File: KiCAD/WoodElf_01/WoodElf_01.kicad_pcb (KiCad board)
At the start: 2 copper layers, 154.3 x 119.4 mm, 164 parts, among them J1 AnalogJoystick, P1 ItsyBitsyM4Express

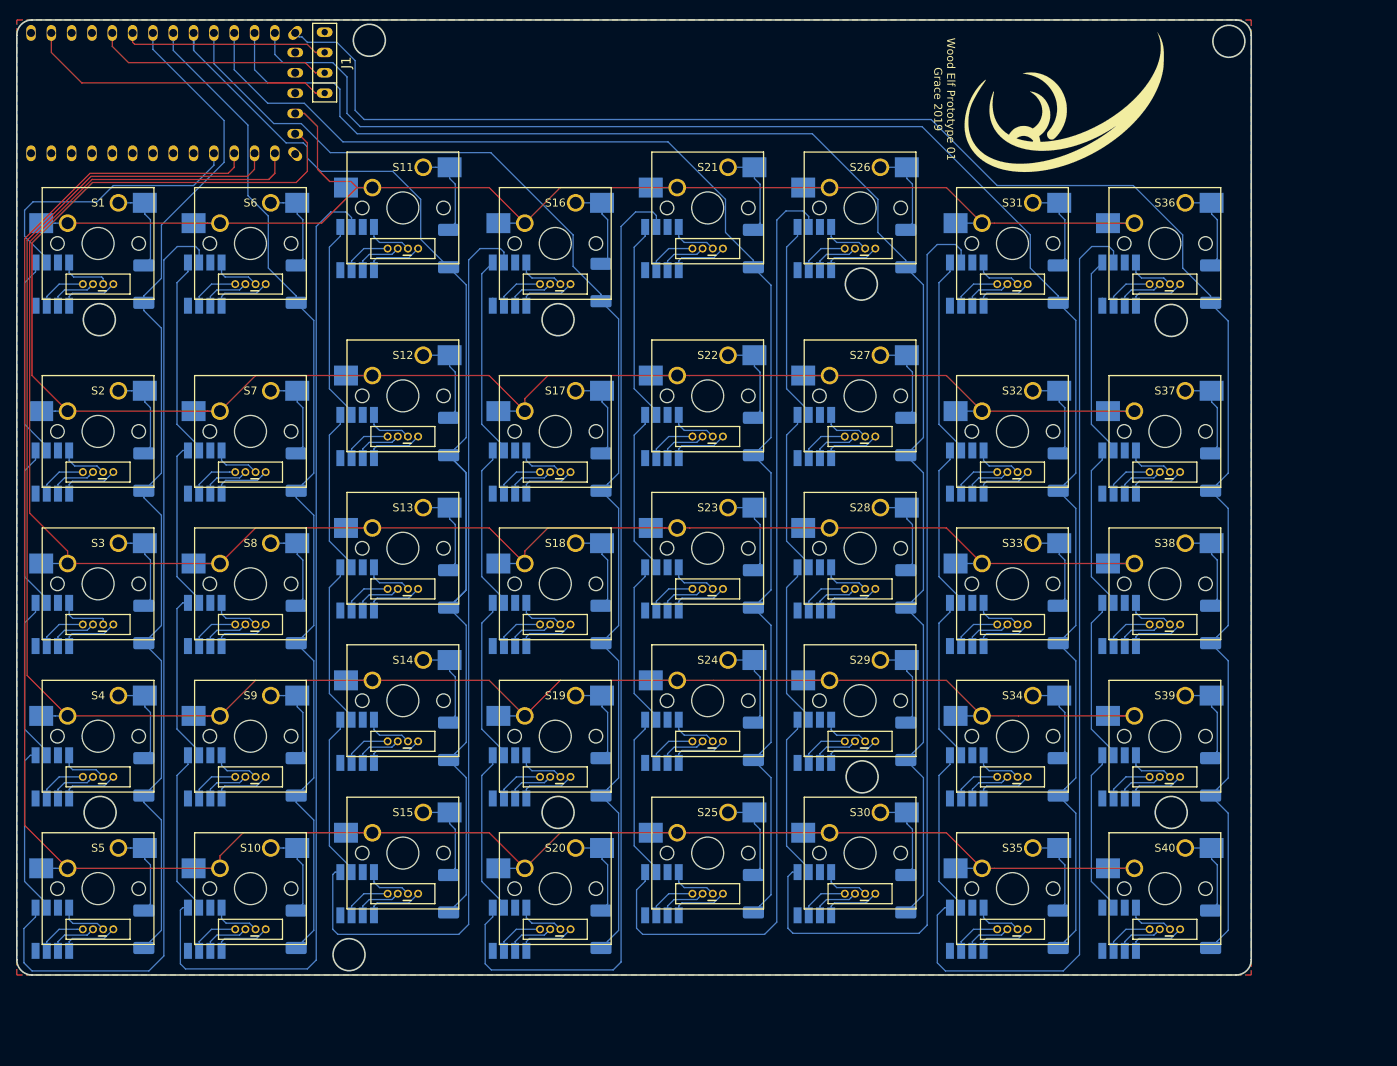
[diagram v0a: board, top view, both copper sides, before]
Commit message: Started on a full-size PCB
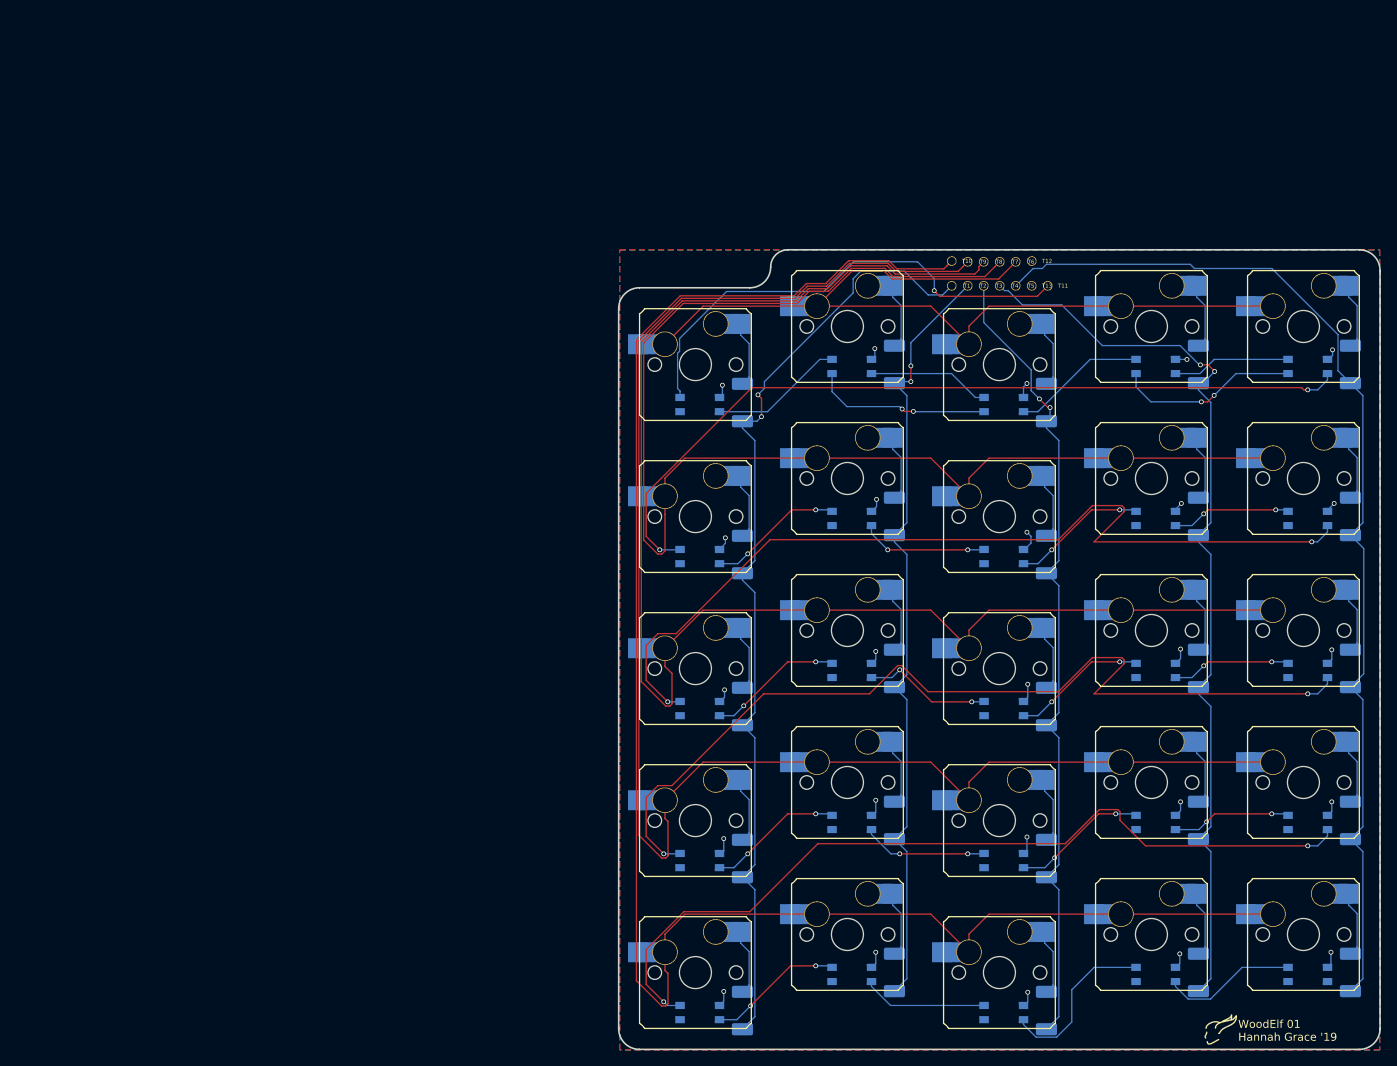
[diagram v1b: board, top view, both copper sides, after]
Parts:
- removed C1, C10, C11, C12, C13, C14, C15, C16, C17, C18, C19, C2, C20, C21, C22, C23, C24, C25, C26, C27, C28, C29, C3, C30, C31, C32, C33, C34, C35, C36, C37, C38, C39, C4, C40, C5, C6, C7, C8, C9: WS2811, WoodElfLib:WS2811
- removed D26, D27, D28, D29, D30, D31, D32, D33, D34, D35, D36, D37, D38, D39, D40: D, Diode_SMD:D_2010_5025Metric_Pad1.52x2.65mm_HandSolder
- removed H26, H27, H28, H29, H30, H31, H32, H33, H34, H35, H36, H37, H38, H39, H40: Kailh_HotSwap_SwitchMount, WoodElfLib:Kailh_HotSwap_Socket
- removed J1: AnalogJoystick, WoodElfLib:Joystick
- removed Logo_2 (x2): Wood Elf, WoodElfLib:WoodElfLogo
- removed P1: ItsyBitsyM4Express, WoodElfLib:ItsyBitsyM4Express
- removed S26, S27, S28, S29, S30, S31, S32, S33, S34, S35, S36, S37, S38, S39, S40: Kailh_RGB_Switch, WoodElfLib:SW_Cherry_MX1A_1.00u_PCB
- added G***: Tiefling_Logo, WoodElf_Lib:Tiefling_Logo, F.Cu at (174.6, 151.2)
- added L1: SK6812MINI, WoodElf_Lib:LED_SK6812MINI_PLCC4_3.5x3.5mm_P1.75mm, F.Cu at (109.5, 72.8)
- added L10: SK6812MINI, WoodElf_Lib:LED_SK6812MINI_PLCC4_3.5x3.5mm_P1.75mm, F.Cu at (109.5, 91.8)
- added L11: SK6812MINI, WoodElf_Lib:LED_SK6812MINI_PLCC4_3.5x3.5mm_P1.75mm, F.Cu at (109.5, 110.8)
- added L12: SK6812MINI, WoodElf_Lib:LED_SK6812MINI_PLCC4_3.5x3.5mm_P1.75mm, F.Cu at (128.5, 106.1)
- added L13: SK6812MINI, WoodElf_Lib:LED_SK6812MINI_PLCC4_3.5x3.5mm_P1.75mm, F.Cu at (147.5, 110.8)
- added L14: SK6812MINI, WoodElf_Lib:LED_SK6812MINI_PLCC4_3.5x3.5mm_P1.75mm, F.Cu at (166.5, 106.1)
- added L15: SK6812MINI, WoodElf_Lib:LED_SK6812MINI_PLCC4_3.5x3.5mm_P1.75mm, F.Cu at (185.5, 106.1)
- added L16: SK6812MINI, WoodElf_Lib:LED_SK6812MINI_PLCC4_3.5x3.5mm_P1.75mm, F.Cu at (185.5, 125.1)
- added L17: SK6812MINI, WoodElf_Lib:LED_SK6812MINI_PLCC4_3.5x3.5mm_P1.75mm, F.Cu at (166.5, 125.1)
- added L18: SK6812MINI, WoodElf_Lib:LED_SK6812MINI_PLCC4_3.5x3.5mm_P1.75mm, F.Cu at (147.5, 129.8)
- added L19: SK6812MINI, WoodElf_Lib:LED_SK6812MINI_PLCC4_3.5x3.5mm_P1.75mm, F.Cu at (128.5, 125.1)
- added L2: SK6812MINI, WoodElf_Lib:LED_SK6812MINI_PLCC4_3.5x3.5mm_P1.75mm, F.Cu at (128.5, 68.1)
- added L20: SK6812MINI, WoodElf_Lib:LED_SK6812MINI_PLCC4_3.5x3.5mm_P1.75mm, F.Cu at (109.5, 129.8)
- added L21: SK6812MINI, WoodElf_Lib:LED_SK6812MINI_PLCC4_3.5x3.5mm_P1.75mm, F.Cu at (109.5, 148.8)
- added L22: SK6812MINI, WoodElf_Lib:LED_SK6812MINI_PLCC4_3.5x3.5mm_P1.75mm, F.Cu at (128.5, 144.1)
- added L23: SK6812MINI, WoodElf_Lib:LED_SK6812MINI_PLCC4_3.5x3.5mm_P1.75mm, F.Cu at (147.5, 148.8)
- added L24: SK6812MINI, WoodElf_Lib:LED_SK6812MINI_PLCC4_3.5x3.5mm_P1.75mm, F.Cu at (166.5, 144.1)
- added L25: SK6812MINI, WoodElf_Lib:LED_SK6812MINI_PLCC4_3.5x3.5mm_P1.75mm, F.Cu at (185.5, 144.1)
- added L3: SK6812MINI, WoodElf_Lib:LED_SK6812MINI_PLCC4_3.5x3.5mm_P1.75mm, F.Cu at (147.5, 72.8)
- added L4: SK6812MINI, WoodElf_Lib:LED_SK6812MINI_PLCC4_3.5x3.5mm_P1.75mm, F.Cu at (166.5, 68.1)
- added L5: SK6812MINI, WoodElf_Lib:LED_SK6812MINI_PLCC4_3.5x3.5mm_P1.75mm, F.Cu at (185.5, 68.1)
- added L6: SK6812MINI, WoodElf_Lib:LED_SK6812MINI_PLCC4_3.5x3.5mm_P1.75mm, F.Cu at (185.5, 87.1)
- added L7: SK6812MINI, WoodElf_Lib:LED_SK6812MINI_PLCC4_3.5x3.5mm_P1.75mm, F.Cu at (166.5, 87.1)
- added L8: SK6812MINI, WoodElf_Lib:LED_SK6812MINI_PLCC4_3.5x3.5mm_P1.75mm, F.Cu at (147.5, 91.8)
- added L9: SK6812MINI, WoodElf_Lib:LED_SK6812MINI_PLCC4_3.5x3.5mm_P1.75mm, F.Cu at (128.5, 87.1)
- added T1: BlankThrough-Hole, WoodElf_Lib:BlankThrough-Hole, F.Cu at (141.0, 58.0)
- added T10: BlankThrough-Hole, WoodElf_Lib:BlankThrough-Hole, F.Cu at (141.0, 54.9)
- added T11: BlankThrough-Hole, WoodElf_Lib:BlankThrough-Hole, F.Cu at (153.0, 58.0)
- added T12: BlankThrough-Hole, WoodElf_Lib:BlankThrough-Hole, F.Cu at (151.0, 54.9)
- added T13: BlankThrough-Hole, WoodElf_Lib:BlankThrough-Hole, F.Cu at (151.0, 58.0)
- added T2: BlankThrough-Hole, WoodElf_Lib:BlankThrough-Hole, F.Cu at (143.0, 58.0)
- added T3: BlankThrough-Hole, WoodElf_Lib:BlankThrough-Hole, F.Cu at (145.0, 58.0)
- added T4: BlankThrough-Hole, WoodElf_Lib:BlankThrough-Hole, F.Cu at (147.0, 58.0)
- added T5: BlankThrough-Hole, WoodElf_Lib:BlankThrough-Hole, F.Cu at (149.0, 58.0)
- added T6: BlankThrough-Hole, WoodElf_Lib:BlankThrough-Hole, F.Cu at (149.0, 55.0)
- added T7: BlankThrough-Hole, WoodElf_Lib:BlankThrough-Hole, F.Cu at (147.0, 55.0)
- added T8: BlankThrough-Hole, WoodElf_Lib:BlankThrough-Hole, F.Cu at (145.0, 55.0)
- added T9: BlankThrough-Hole, WoodElf_Lib:BlankThrough-Hole, F.Cu at (143.0, 55.0)
- D1, D10, D11, D12, D13, D14, D15, D16, D17, D18, D19, D2, D20, D21, D22, D23, D24, D25, D3, D4, D5, D6, D7, D8, D9: value D -> DIODE; footprint WoodElfLib:D_2010_5025Metric_Pad1.52x2.65mm_HandSolder -> Diode_SMD:D_2010_5025Metric_Pad1.52x2.65mm_HandSolder
- H1, H10, H11, H12, H13, H14, H15, H16, H17, H18, H19, H2, H20, H21, H22, H23, H24, H25, H3, H4, H5, H6, H7, H8, H9: footprint WoodElfLib:Kailh_HotSwap_Socket -> WoodElf_Lib:Kailh_HotSwap_Socket
- S1, S10, S11, S12, S13, S14, S15, S16, S17, S18, S19, S2, S20, S21, S22, S23, S24, S25, S3, S4, S5, S6, S7, S8, S9: footprint WoodElfLib:SW_Cherry_MX1A_1.00u_PCB -> WoodElf_Lib:SW_Cherry_MX1A_1.00u_PCB
- moved D5 166.5 mm to (190.8, 67.8), turned to 270 degrees
- moved H5 166.3 mm to (187.5, 58.0)
- moved S5 166.3 mm to (187.5, 58.0)
- moved D4 141.6 mm to (171.8, 67.8), turned to 270 degrees
- moved H4 141.3 mm to (168.5, 58.0)
- moved S4 141.3 mm to (168.5, 58.0)
- moved D6 134.9 mm to (190.8, 86.8), turned to 270 degrees
- moved H6 134.9 mm to (187.5, 77.0)
- moved S6 134.9 mm to (187.5, 77.0)
- moved D15 116.2 mm to (190.8, 105.8), turned to 270 degrees
- moved D3 116.2 mm to (152.8, 72.6), turned to 270 degrees
- moved H15 116.0 mm to (187.5, 96.0)
- moved S15 116.0 mm to (187.5, 96.0)
- moved H3 116.0 mm to (149.5, 62.8)
- moved S3 116.0 mm to (149.5, 62.8)
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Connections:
- D1 pad 1: /A2 -> Net-(D1-Pad1)
- D1 pad 2: Net-(D1-Pad2) -> /Col2
- D10 pad 1: /A3 -> Net-(D10-Pad1)
- D10 pad 2: Net-(D10-Pad2) -> /Col1
- D11 pad 1: /A4 -> Net-(D11-Pad1)
- D11 pad 2: Net-(D11-Pad2) -> /Col1
- D12 pad 1: /A4 -> Net-(D12-Pad1)
- D12 pad 2: Net-(D12-Pad2) -> /Col2
- D13 pad 1: /A4 -> Net-(D13-Pad1)
- D13 pad 2: Net-(D13-Pad2) -> /Col3
- D14 pad 1: /A4 -> Net-(D14-Pad1)
- D14 pad 2: Net-(D14-Pad2) -> /Col4
- D15 pad 1: /A4 -> Net-(D15-Pad1)
- D15 pad 2: Net-(D15-Pad2) -> /Col5
- D16 pad 1: /A5 -> Net-(D16-Pad1)
- D16 pad 2: Net-(D16-Pad2) -> /Col5
- D17 pad 1: /A5 -> Net-(D17-Pad1)
- D17 pad 2: Net-(D17-Pad2) -> /Col4
- D18 pad 1: /A5 -> Net-(D18-Pad1)
- D18 pad 2: Net-(D18-Pad2) -> /Col3
- D19 pad 1: /A5 -> Net-(D19-Pad1)
- D19 pad 2: Net-(D19-Pad2) -> /Col2
- D2 pad 1: /A2 -> Net-(D2-Pad1)
- D2 pad 2: Net-(D2-Pad2) -> /Col1
- D20 pad 1: /A5 -> Net-(D20-Pad1)
- D20 pad 2: Net-(D20-Pad2) -> /Col1
- D21 pad 1: /SCK -> Net-(D21-Pad1)
- D21 pad 2: Net-(D21-Pad2) -> /Col1
- D22 pad 1: /SCK -> Net-(D22-Pad1)
- D22 pad 2: Net-(D22-Pad2) -> /Col2
- D23 pad 1: /SCK -> Net-(D23-Pad1)
- D23 pad 2: Net-(D23-Pad2) -> /Col3
- D24 pad 1: /SCK -> Net-(D24-Pad1)
- D24 pad 2: Net-(D24-Pad2) -> /Col4
- D25 pad 1: /SCK -> Net-(D25-Pad1)
- D25 pad 2: Net-(D25-Pad2) -> /Col5
- D3 pad 1: /A2 -> Net-(D3-Pad1)
- D3 pad 2: Net-(D3-Pad2) -> /Col3
- D4 pad 1: /A2 -> Net-(D4-Pad1)
- D4 pad 2: Net-(D4-Pad2) -> /Col4
- D5 pad 1: /A2 -> Net-(D5-Pad1)
- D5 pad 2: Net-(D5-Pad2) -> /Col5
- D6 pad 1: /A3 -> Net-(D6-Pad1)
- D6 pad 2: Net-(D6-Pad2) -> /Col5
- D7 pad 1: /A3 -> Net-(D7-Pad1)
- D7 pad 2: Net-(D7-Pad2) -> /Col4
- D8 pad 1: /A3 -> Net-(D8-Pad1)
- D8 pad 2: Net-(D8-Pad2) -> /Col3
- D9 pad 1: /A3 -> Net-(D9-Pad1)
- D9 pad 2: Net-(D9-Pad2) -> /Col2
- H1 pad 1: Net-(D2-Pad2) -> Net-(D2-Pad1)
- H1 pad 2: /GPIO#3 -> /Row1
- H10 pad 1: Net-(D10-Pad2) -> Net-(D10-Pad1)
- H10 pad 2: /SCL -> /Row2
- H11 pad 1: Net-(D11-Pad2) -> Net-(D11-Pad1)
- H11 pad 2: /GPIO#3 -> /Row3
- H12 pad 1: Net-(D12-Pad2) -> Net-(D12-Pad1)
- H12 pad 2: /GPIO#4 -> /Row3
- H13 pad 1: Net-(D13-Pad2) -> Net-(D13-Pad1)
- H13 pad 2: /GPIO#1 -> /Row3
- H14 pad 1: Net-(D14-Pad2) -> Net-(D14-Pad1)
- H14 pad 2: /SDA -> /Row3
- H15 pad 1: Net-(D15-Pad2) -> Net-(D15-Pad1)
- H15 pad 2: /SCL -> /Row3
- H16 pad 1: Net-(D16-Pad2) -> Net-(D16-Pad1)
- H16 pad 2: /GPIO#3 -> /Row4
- H17 pad 1: Net-(D17-Pad2) -> Net-(D17-Pad1)
- H17 pad 2: /GPIO#4 -> /Row4
- H18 pad 1: Net-(D18-Pad2) -> Net-(D18-Pad1)
- H18 pad 2: /GPIO#1 -> /Row4
- H19 pad 1: Net-(D19-Pad2) -> Net-(D19-Pad1)
- H19 pad 2: /SDA -> /Row4
- H2 pad 1: Net-(D1-Pad2) -> Net-(D1-Pad1)
- H2 pad 2: /GPIO#4 -> /Row1
- H20 pad 1: Net-(D20-Pad2) -> Net-(D20-Pad1)
- H20 pad 2: /SCL -> /Row4
- H21 pad 1: Net-(D21-Pad2) -> Net-(D21-Pad1)
- H21 pad 2: /GPIO#3 -> /Row5
- H22 pad 1: Net-(D22-Pad2) -> Net-(D22-Pad1)
- H22 pad 2: /GPIO#4 -> /Row5
- H23 pad 1: Net-(D23-Pad2) -> Net-(D23-Pad1)
- H23 pad 2: /GPIO#1 -> /Row5
- H24 pad 1: Net-(D24-Pad2) -> Net-(D24-Pad1)
- H24 pad 2: /SDA -> /Row5
- H25 pad 1: Net-(D25-Pad2) -> Net-(D25-Pad1)
- H25 pad 2: /SCL -> /Row5
- H3 pad 1: Net-(D3-Pad2) -> Net-(D3-Pad1)
- H3 pad 2: /GPIO#1 -> /Row1
- H4 pad 1: Net-(D4-Pad2) -> Net-(D4-Pad1)
- H4 pad 2: /SDA -> /Row1
- H5 pad 1: Net-(D5-Pad2) -> Net-(D5-Pad1)
- H5 pad 2: /SCL -> /Row1
- H6 pad 1: Net-(D6-Pad2) -> Net-(D6-Pad1)
- H6 pad 2: /GPIO#3 -> /Row2
- H7 pad 1: Net-(D7-Pad2) -> Net-(D7-Pad1)
- H7 pad 2: /GPIO#4 -> /Row2
- H8 pad 1: Net-(D8-Pad2) -> Net-(D8-Pad1)
- H8 pad 2: /GPIO#1 -> /Row2
- H9 pad 1: Net-(D9-Pad2) -> Net-(D9-Pad1)
- H9 pad 2: /SDA -> /Row2
- S1 pad 1: Net-(D2-Pad2) -> Net-(D2-Pad1)
- S1 pad 2: /GPIO#3 -> /Row1
- S10 pad 1: Net-(D10-Pad2) -> Net-(D10-Pad1)
- S10 pad 2: /SCL -> /Row2
- S11 pad 1: Net-(D11-Pad2) -> Net-(D11-Pad1)
- S11 pad 2: /GPIO#3 -> /Row3
- S12 pad 1: Net-(D12-Pad2) -> Net-(D12-Pad1)
- S12 pad 2: /GPIO#4 -> /Row3
- S13 pad 1: Net-(D13-Pad2) -> Net-(D13-Pad1)
- S13 pad 2: /GPIO#1 -> /Row3
- S14 pad 1: Net-(D14-Pad2) -> Net-(D14-Pad1)
- S14 pad 2: /SDA -> /Row3
- S15 pad 1: Net-(D15-Pad2) -> Net-(D15-Pad1)
- S15 pad 2: /SCL -> /Row3
- S16 pad 1: Net-(D16-Pad2) -> Net-(D16-Pad1)
- S16 pad 2: /GPIO#3 -> /Row4
- S17 pad 1: Net-(D17-Pad2) -> Net-(D17-Pad1)
- S17 pad 2: /GPIO#4 -> /Row4
- S18 pad 1: Net-(D18-Pad2) -> Net-(D18-Pad1)
- S18 pad 2: /GPIO#1 -> /Row4
- S19 pad 1: Net-(D19-Pad2) -> Net-(D19-Pad1)
- S19 pad 2: /SDA -> /Row4
- S2 pad 1: Net-(D1-Pad2) -> Net-(D1-Pad1)
- S2 pad 2: /GPIO#4 -> /Row1
- S20 pad 1: Net-(D20-Pad2) -> Net-(D20-Pad1)
- S20 pad 2: /SCL -> /Row4
- S21 pad 1: Net-(D21-Pad2) -> Net-(D21-Pad1)
- S21 pad 2: /GPIO#3 -> /Row5
- S22 pad 1: Net-(D22-Pad2) -> Net-(D22-Pad1)
- S22 pad 2: /GPIO#4 -> /Row5
- S23 pad 1: Net-(D23-Pad2) -> Net-(D23-Pad1)
- S23 pad 2: /GPIO#1 -> /Row5
- S24 pad 1: Net-(D24-Pad2) -> Net-(D24-Pad1)
- S24 pad 2: /SDA -> /Row5
- S25 pad 1: Net-(D25-Pad2) -> Net-(D25-Pad1)
- S25 pad 2: /SCL -> /Row5
- S3 pad 1: Net-(D3-Pad2) -> Net-(D3-Pad1)
- S3 pad 2: /GPIO#1 -> /Row1
- S4 pad 1: Net-(D4-Pad2) -> Net-(D4-Pad1)
- S4 pad 2: /SDA -> /Row1
- S5 pad 1: Net-(D5-Pad2) -> Net-(D5-Pad1)
- S5 pad 2: /SCL -> /Row1
- S6 pad 1: Net-(D6-Pad2) -> Net-(D6-Pad1)
- S6 pad 2: /GPIO#3 -> /Row2
- S7 pad 1: Net-(D7-Pad2) -> Net-(D7-Pad1)
- S7 pad 2: /GPIO#4 -> /Row2
- S8 pad 1: Net-(D8-Pad2) -> Net-(D8-Pad1)
- S8 pad 2: /GPIO#1 -> /Row2
- S9 pad 1: Net-(D9-Pad2) -> Net-(D9-Pad1)
- S9 pad 2: /SDA -> /Row2
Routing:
- net /SCL: track 280.6 -> 0.00 mm
- net /SDA: track 262.8 -> 0.00 mm
- net /GPIO#1: track 246.9 -> 0.00 mm
- net /USB_1: track 245.3 -> 0.00 mm
- net /Row5: track 0.00 -> 237.8 mm
- net /GPIO#4: track 234.6 -> 0.00 mm
- net /GPIO#2: track 222.8 -> 0.00 mm
- net /Row4: track 0.00 -> 220.0 mm
- net /MI: track 207.0 -> 0.00 mm
- net /Row3: track 0.00 -> 203.1 mm
- net /MO: track 189.1 -> 0.00 mm
- net /Row2: track 0.00 -> 186.0 mm
- net /GPIO#3: track 181.8 -> 0.00 mm
- net /SCK: track 170.6 -> 0.00 mm
- net /A4: track 161.6 -> 0.00 mm
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- added copper zone on F.Cu, net VDD
- added copper zone on B.Cu, net VSS
- removed copper zone on B.Cu, net /GND_1
- removed copper zone on F.Cu, net /USB_1
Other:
- board size 154.3 x 119.4 mm -> 95.2 x 100 mm
- board text added: "WoodElf 01 Hannah Grace '19"
- board text removed: "Wood Elf Prototype 01 Grace 2019"
